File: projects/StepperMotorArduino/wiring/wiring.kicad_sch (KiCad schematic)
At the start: 18 parts, among them J1 Conn_01x02_Pin, J2 Conn_01x02_Pin, J3 Conn_01x02_Pin, J4 Conn_01x02_Pin, J5 Conn_01x04_Pin, J6 Conn_01x04_Pin, J7 Conn_01x02_Pin, M1 Stepper_Motor_bipolar, M2 Stepper_Motor_bipolar, SW1 Limit switch (top), SW2 Limit switch (bottom), SW3 Limit switch (right), SW4 Limit switch (left), U1 NRF24L01_Breakout

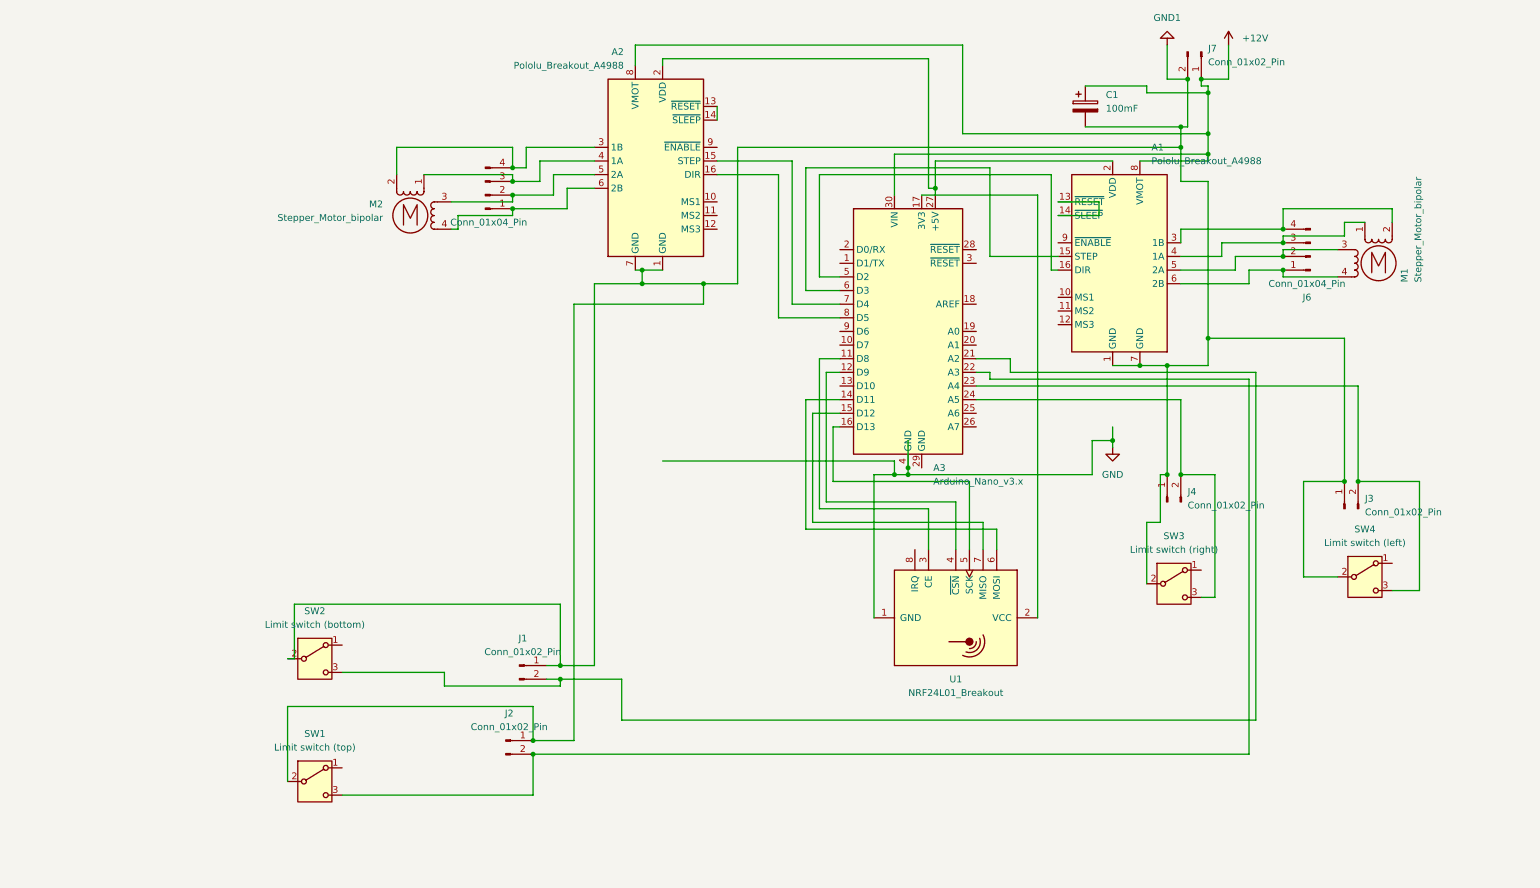
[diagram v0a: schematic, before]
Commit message: Progress
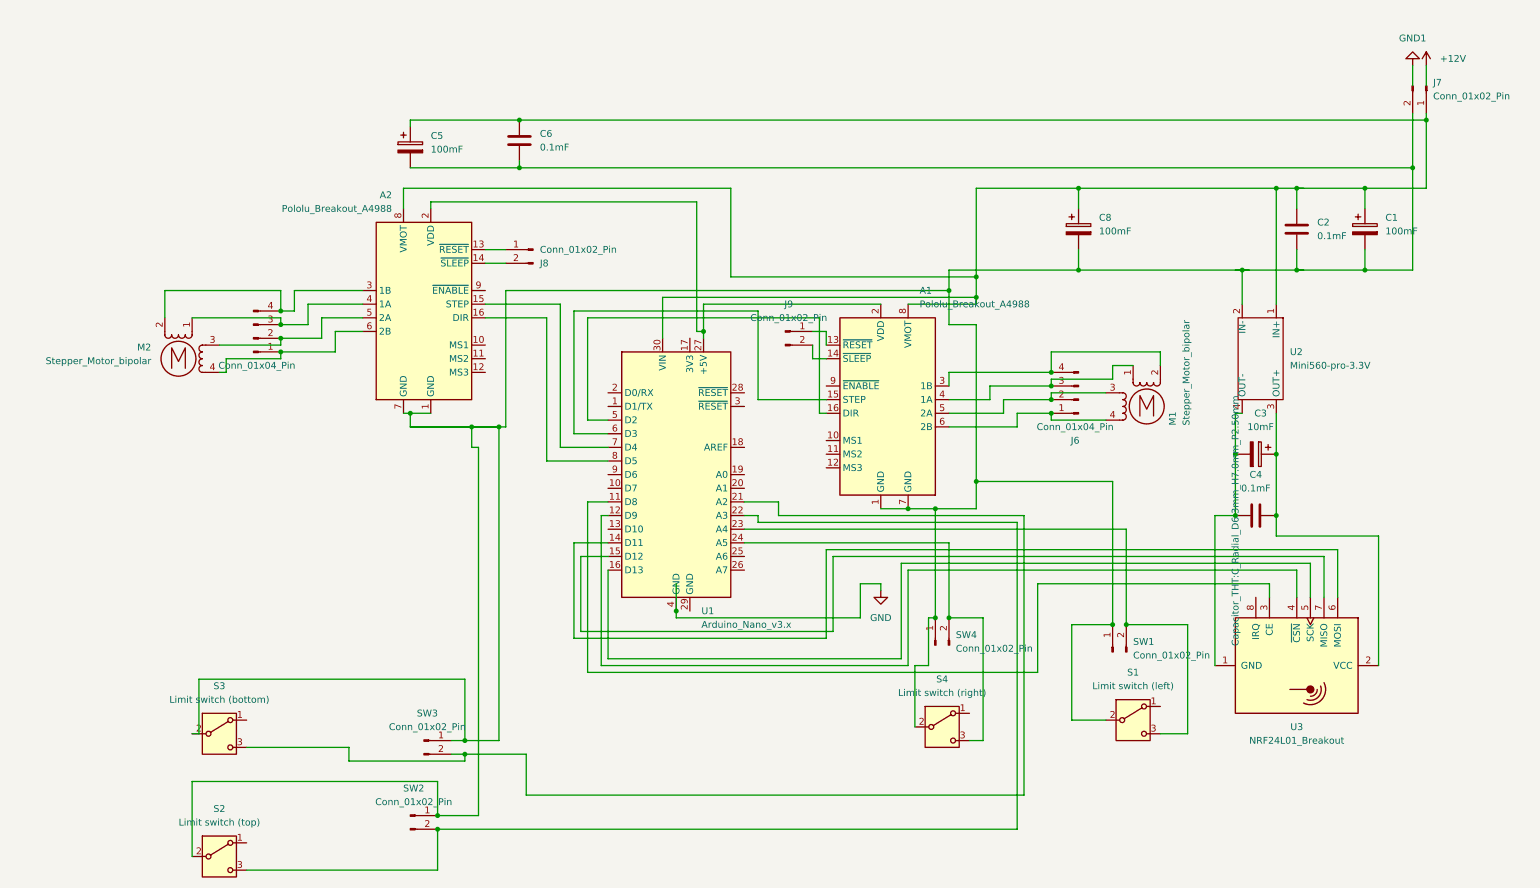
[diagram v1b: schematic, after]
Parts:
- removed U1: NRF24L01_Breakout, RF_Module:nRF24L01_Breakout, symbol RF:NRF24L01_Breakout
- added C2, C4, C6: 0.1mF, Capacitor_THT:C_Radial_D6.3mm_H7.0mm_P2.50mm, symbol Device:C
- added C3: 10mF, Capacitor_THT:CP_Radial_D8.0mm_P3.80mm, symbol Device:C_Polarized
- added C5, C8: 100mF, Capacitor_THT:CP_Radial_D8.0mm_P3.80mm, symbol Device:C_Polarized
- added J8, J9: Conn_01x02_Pin, Connector_PinSocket_2.54mm:PinSocket_1x02_P2.54mm_Vertical, symbol Connector:Conn_01x02_Pin
- added U2: Mini560-pro-3.3V, custom:Mini560-pro-3.3V, symbol custom_stuff:Mini560-pro-3.3V
- added U3: NRF24L01_Breakout, RF_Module:nRF24L01_Breakout, symbol RF:NRF24L01_Breakout
- C1: footprint Capacitor_SMD:C_0201_0603Metric -> Capacitor_THT:CP_Radial_D8.0mm_P3.80mm
- renumbered SW4 to S1, SW1 to S2, SW2 to S3, SW3 to S4, J3 to SW1, J2 to SW2, J1 to SW3, J4 to SW4, A3 to U1
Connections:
- net +12V: no longer A1.8 (VMOT), A2.8 (VMOT), C1.1, J7.1 (Pin_1), U1.30 (VIN)
- net GND1: no longer A1.1 (GND), A1.7 (GND), A2.1 (GND), A2.7 (GND), C1.2, J7.2 (Pin_2), S1.2 (B), S2.2 (B), S3.2 (B), S4.2 (B), SW1.1 (Pin_1), SW2.1 (Pin_1), SW3.1 (Pin_1), SW4.1 (Pin_1)
- net at U1.11 (D8): now also U3.3 (CE)
- net at U1.12 (D9): now also U3.4 (~{CSN})
- net at U1.14 (D11): now also U3.6 (MOSI)
- net at U1.15 (D12): now also U3.7 (MISO)
- net at U1.16 (D13): now also U3.5 (SCK)
- net at A1.13 (~{RESET}): now also J9.1 (Pin_1); no longer A1.14 (~{SLEEP})
- net at A2.13 (~{RESET}): now also J8.1 (Pin_1); no longer A2.14 (~{SLEEP})
- new net: A1.8 (VMOT), A2.8 (VMOT), C1.1, C2.1, C5.1, C6.1, C8.1, J7.1 (Pin_1), U1.30 (VIN), U2.1 (IN+)
- new net: A1.1 (GND), A1.7 (GND), A2.1 (GND), A2.7 (GND), C1.2, C2.2, C5.2, C6.2, C8.2, J7.2 (Pin_2), S1.2 (B), S2.2 (B), S3.2 (B), S4.2 (B), SW1.1 (Pin_1), SW2.1 (Pin_1), SW3.1 (Pin_1), SW4.1 (Pin_1), U2.2 (IN-)
- new net: C3.1, C4.1, U2.3 (OUT+), U3.2 (VCC)
- new net: C3.2, C4.2, U2.4 (OUT-), U3.1 (GND)
- new net: A1.14 (~{SLEEP}), J9.2 (Pin_2)
- new net: A2.14 (~{SLEEP}), J8.2 (Pin_2)
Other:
- moved on the sheet: A1, A2, C1, J6, J7, M1, M2, S1, S2, S3, S4, SW1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

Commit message: Fixes
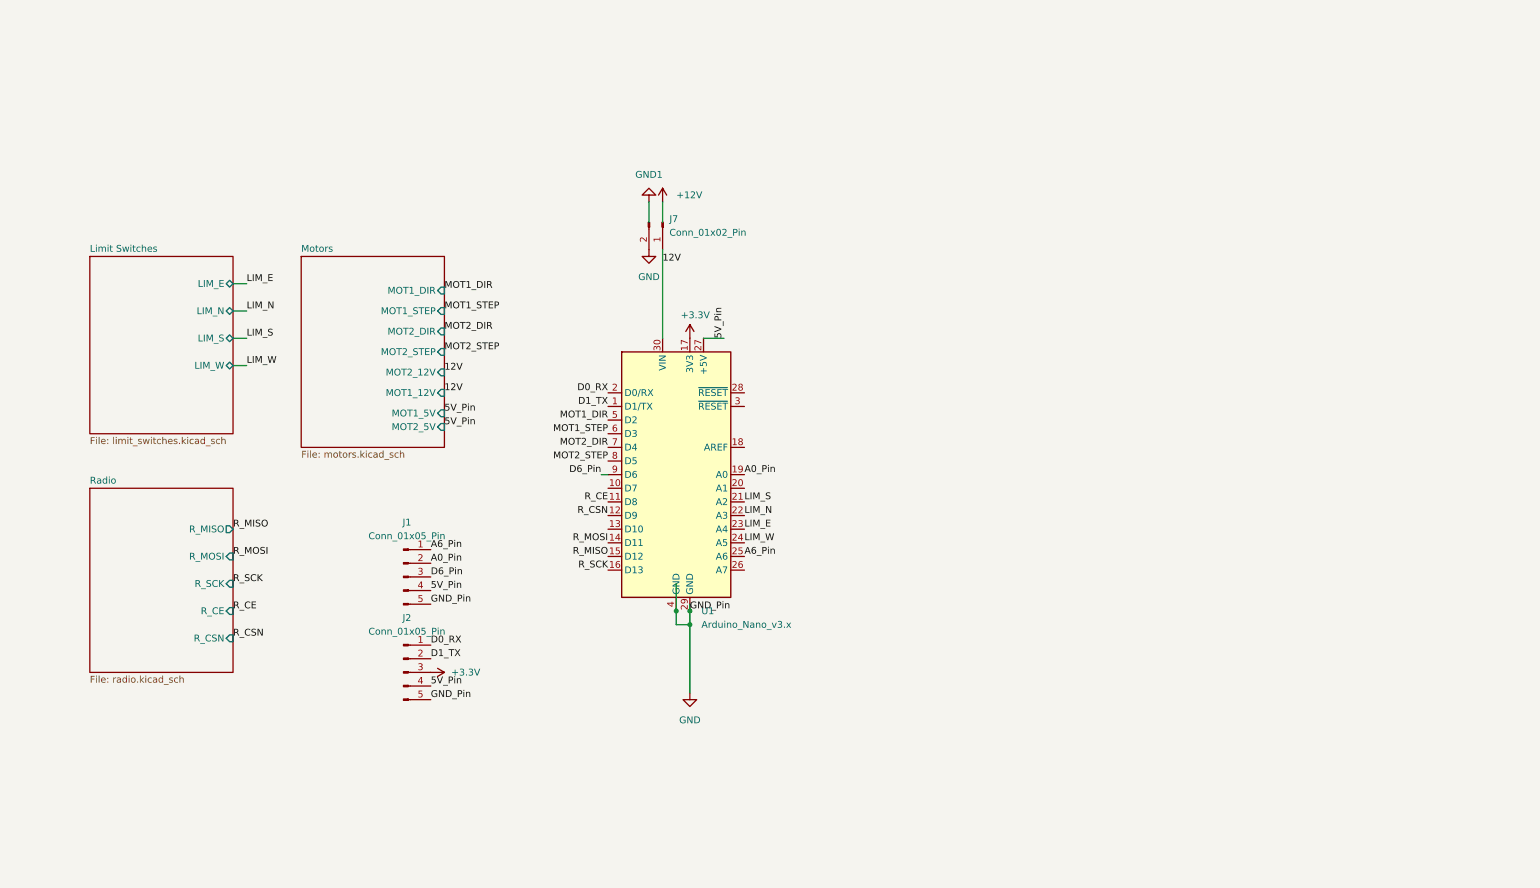
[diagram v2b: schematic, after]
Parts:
- removed A1, A2: Pololu_Breakout_A4988, Module:Pololu_Breakout-16_15.2x20.3mm, symbol Driver_Motor:Pololu_Breakout_A4988
- removed C1, C5, C8: 100mF, Capacitor_THT:CP_Radial_D8.0mm_P3.80mm, symbol Device:C_Polarized
- removed C2, C4, C6: 0.1mF, Capacitor_THT:C_Radial_D6.3mm_H7.0mm_P2.50mm, symbol Device:C
- removed C3: 10mF, Capacitor_THT:CP_Radial_D8.0mm_P3.80mm, symbol Device:C_Polarized
- removed J5, J6: Conn_01x04_Pin, Connector_PinHeader_2.54mm:PinHeader_1x04_P2.54mm_Vertical, symbol Connector:Conn_01x04_Pin
- removed J8, J9, SW1, SW2, SW3, SW4: Conn_01x02_Pin, Connector_PinSocket_2.54mm:PinSocket_1x02_P2.54mm_Vertical, symbol Connector:Conn_01x02_Pin
- removed M1, M2: Stepper_Motor_bipolar, symbol Motor:Stepper_Motor_bipolar
- removed S1: Limit switch (left), symbol Switch:SW_SPDT
- removed S2: Limit switch (top), symbol Switch:SW_SPDT
- removed S3: Limit switch (bottom), symbol Switch:SW_SPDT
- removed S4: Limit switch (right), symbol Switch:SW_SPDT
- removed U2: Mini560-pro-3.3V, custom:Mini560-pro-3.3V, symbol custom_stuff:Mini560-pro-3.3V
- removed U3: NRF24L01_Breakout, RF_Module:nRF24L01_Breakout, symbol RF:NRF24L01_Breakout
- added J1, J2: Conn_01x05_Pin, Connector_PinSocket_2.54mm:PinSocket_1x05_P2.54mm_Vertical, symbol Connector:Conn_01x05_Pin
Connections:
- net GND: now also J7.2 (Pin_2), U1.29 (GND), J1.5 (Pin_5), J2.5 (Pin_5)
- net 12V: now reaches J7.1 (Pin_1), U1.30 (VIN)
- net D1_TX: now reaches U1.1 (D1/TX)
- net D1_TX: now also J2.2 (Pin_2)
- net R_CE: now reaches U1.11 (D8)
- net R_CSN: now reaches U1.12 (D9)
- net R_MOSI: now reaches U1.14 (D11)
- net R_MISO: now reaches U1.15 (D12)
- net R_SCK: now reaches U1.16 (D13)
- net +3.3V: now reaches U1.17 (3V3)
- net +3.3V: now also J2.3 (Pin_3)
- net A0_Pin: now reaches U1.19 (A0)
- net A0_Pin: now also J1.2 (Pin_2)
- net D0_RX: now reaches U1.2 (D0/RX)
- net D0_RX: now also J2.1 (Pin_1)
- net LIM_S: now reaches U1.21 (A2)
- net LIM_N: now reaches U1.22 (A3)
- net LIM_E: now reaches U1.23 (A4)
- net LIM_W: now reaches U1.24 (A5)
- net A6_Pin: now reaches U1.25 (A6)
- net A6_Pin: now also J1.1 (Pin_1)
- net 5V_Pin: now reaches U1.27 (+5V)
- net 5V_Pin: now also J1.4 (Pin_4), J2.4 (Pin_4)
- net MOT1_DIR: now reaches U1.5 (D2)
- net MOT1_STEP: now reaches U1.6 (D3)
- net MOT2_DIR: now reaches U1.7 (D4)
- net MOT2_STEP: now reaches U1.8 (D5)
- net D6_Pin: now reaches U1.9 (D6)
- net D6_Pin: now also J1.3 (Pin_3)
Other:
- added sheet Limit Switches (limit_switches.kicad_sch)
- added sheet Motors (motors.kicad_sch)
- added sheet Radio (radio.kicad_sch)
- moved on the sheet: J7
